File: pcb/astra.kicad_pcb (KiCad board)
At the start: 4 copper layers, 49.2 x 45.5 mm, 89 parts, among them J1 Conn_01x02_Pin, J2 Conn_01x24_MountingPin, J3 Conn_02x04_Odd_Even, J4 Conn_02x05_Odd_Even, M1 Motor_DC, M2 Motor_DC, M3 Motor_DC, M4 Motor_DC, Q1 AO3400A, Q2 AO3400A, Q3 AO3400A, Q4 AO3400A, SW1 SS-3235S-L1, SW2 SW_Push, U1 TLV1117LV33DCYR, U2 W25Q64JVSSIQ_C179171, U3 STM32H750VBTx, U4 TLV74328PDBVR, U5 NRF24L01_Breakout, U6 TLV74315PDBVR, U7 BMI270, U8 HYCW110-TF10-180B, X1 OT322524MJBA4SL, Y1 25 MHz

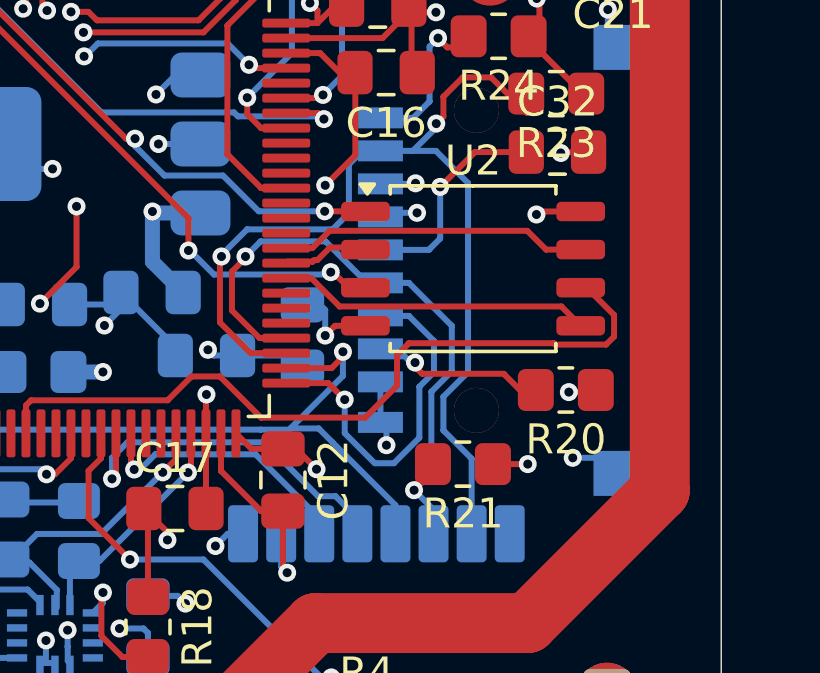
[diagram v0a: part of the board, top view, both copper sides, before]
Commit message: [pcb] controller schematic, intial layout
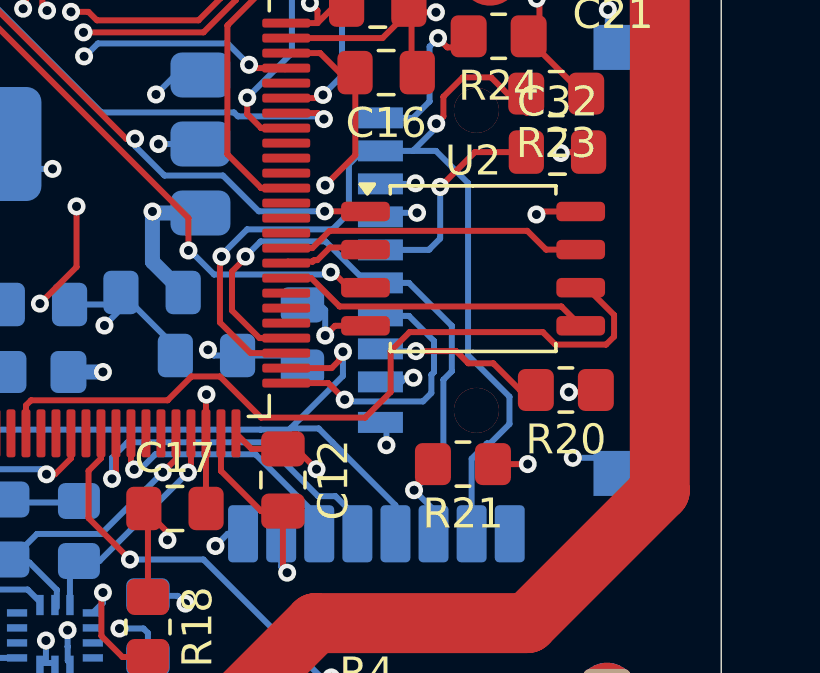
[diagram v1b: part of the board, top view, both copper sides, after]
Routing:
- net CS_SD: track 12.1 -> 9.11 mm
- net QSPI_CLK: track 25.5 -> 26.0 mm
- net GND: track 126.6 -> 126.4 mm, vias 38 -> 39
